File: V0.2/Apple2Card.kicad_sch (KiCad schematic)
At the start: 61 parts, among them J1 Conn_01x08_Pin, P2 Conn_02x13_Top_Bottom, Q2 2N3904, SW1 SW_DIP_x08, U1C1 74LS240, U1E1 74LS14, U2 74LS133, U2B1 74LS08, U2D1 74LS138, U2E1 74LS08, U3A1 2764, U3C1 ATF16V8C, U3D1 ATF16V8C, U3E1 74LS273/74HCT273, U4E1 74LS245, U5A1 NCR5380, U5C1 6264, U5E1 74LS14, U6C1 74LS32, U6D1 74LS74, U6E1 74LS74

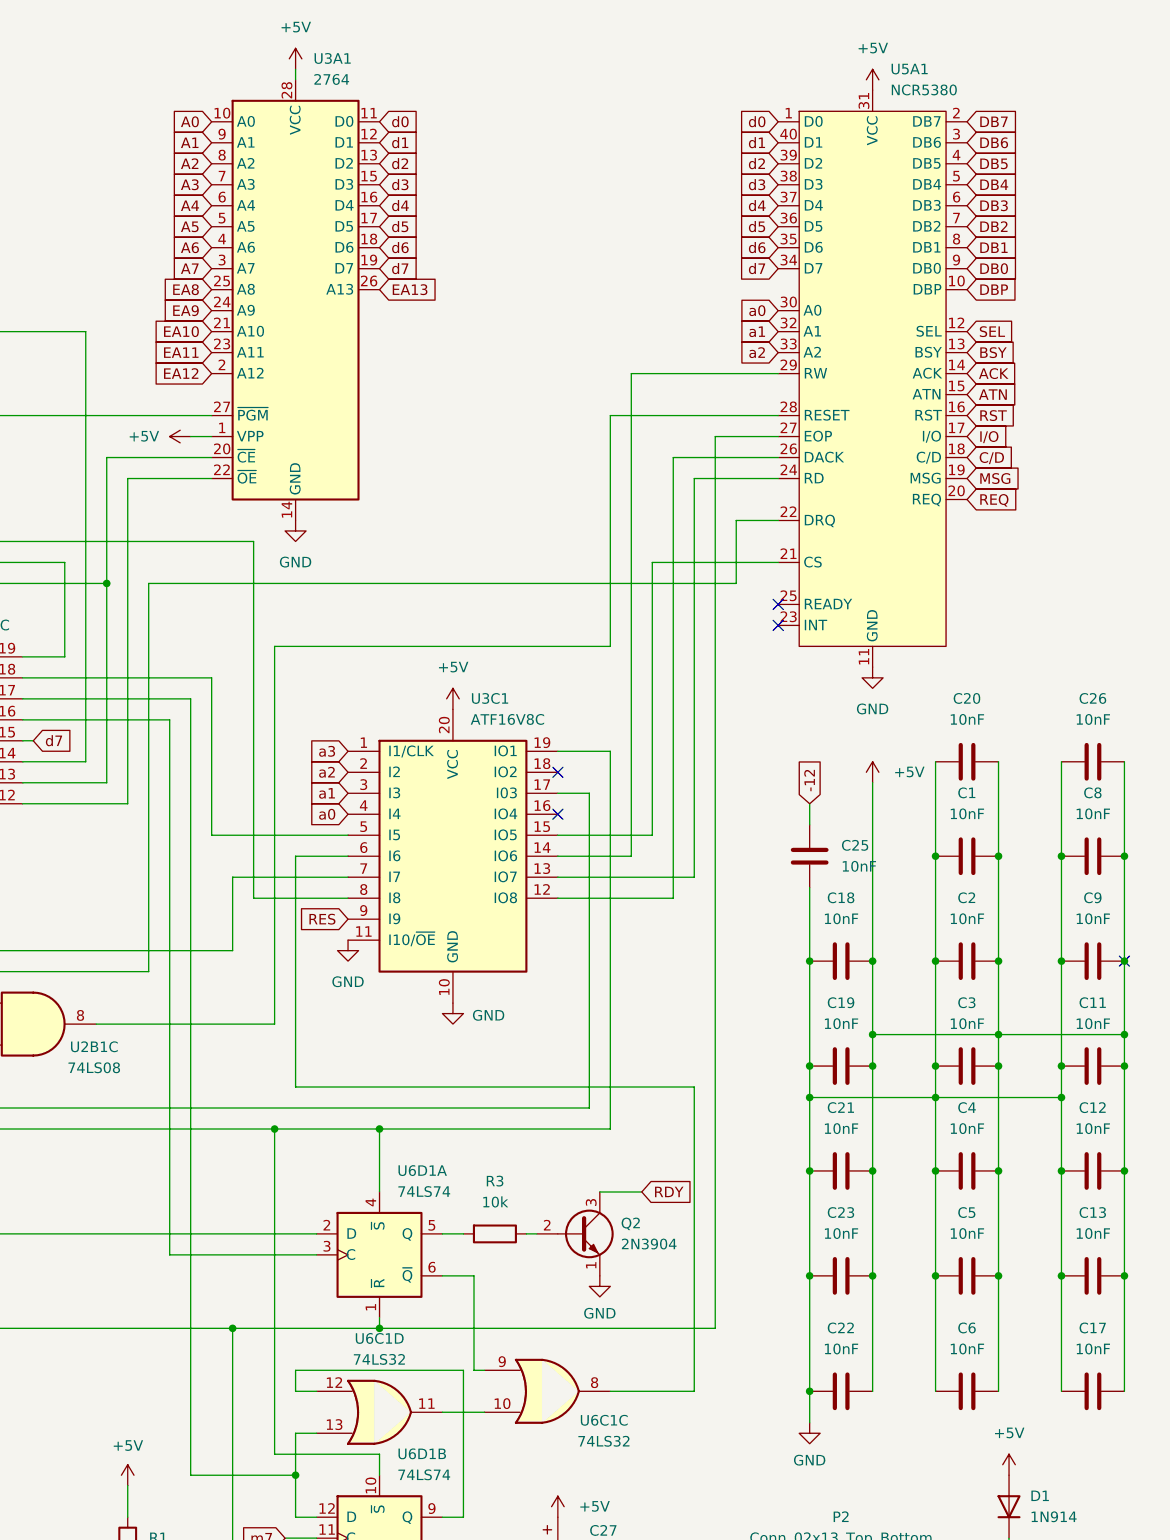
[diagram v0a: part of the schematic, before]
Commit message: menage
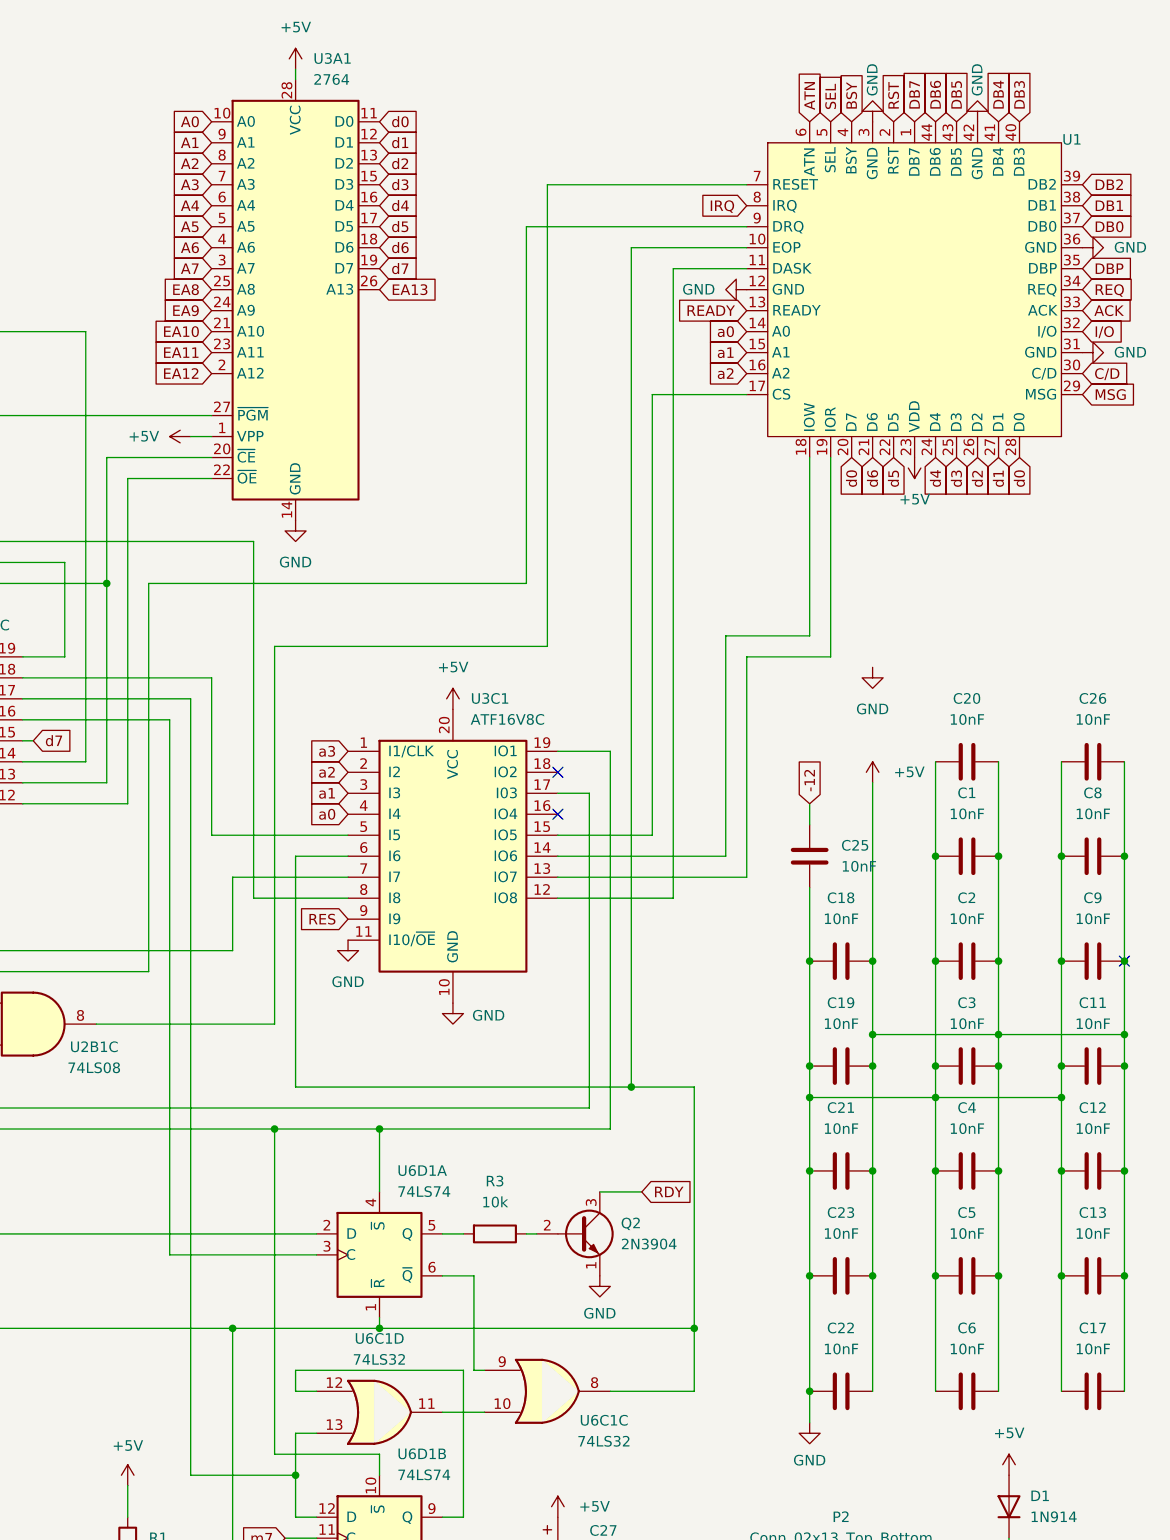
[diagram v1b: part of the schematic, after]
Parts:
- removed U5A1: NCR5380, Package_DIP:DIP-40_W15.24mm, symbol ncr5380:NCR5880
- added U1: ~, Package_LCC:PLCC-44, symbol 53c80:53c80_PLCC
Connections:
- net +5V: now also U1.23 (VDD)
- net ACK: now also U1.33 (ACK)
- net ATN: now also U1.6 (ATN)
- net BSY: now also U1.4 (BSY)
- net C/D: now also U1.30 (C/D)
- net DB0: now also U1.37 (DB0)
- net DB1: now also U1.38 (DB1)
- net DB2: now also U1.39 (DB2)
- net DB3: now also U1.40 (DB3)
- net DB4: now also U1.41 (DB4)
- net DB5: now also U1.43 (DB5)
- net DB6: now also U1.44 (DB6)
- net DB7: now also U1.1 (DB7)
- net DBP: now also U1.35 (DBP)
- net GND: now also U1.12 (GND), U1.3 (GND), U1.31 (GND), U1.36 (GND), U1.42 (GND)
- net IRQ: now also U1.8 (IRQ)
- net I/O: now also U1.32 (I/O)
- net MSG: now also U1.29 (MSG)
- net REQ: now also U1.34 (REQ)
- net RST: now also U1.2 (RST)
- net SEL: now also U1.5 (SEL)
- net a0: now also U1.14 (A0)
- net a1: now also U1.15 (A1)
- net a2: now also U1.16 (A2)
- net d0: now also U1.20 (D7), U1.28 (D0)
- net d1: now also U1.27 (D1)
- net d2: now also U1.26 (D2)
- net d3: now also U1.25 (D3)
- net d4: now also U1.24 (D4)
- net d5: now also U1.22 (D5)
- net d6: now also U1.21 (D6)
- net at R1.2, U6D1.1 (~{R}), U6D1.13 (~{R})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: now also U3C1.6 (I6), U6C1.8, U1.10 (EOP)
- net at U3C1.15 (IO5): now also U1.17 (CS)
- net at U3D1.9 (I9), U6D1.2 (D): now also U1.9 (DRQ)
- net at U3C1.13 (IO7): now also U1.19 (IOR)
- net at U3C1.12 (IO8): now also U1.11 (DASK)
- net at U2B1.8: now also U1.7 (RESET)
- net at U3C1.14 (IO6): now also U1.18 (IOW)
- new net READY: U1.13 (READY)
- no-connect marks 17 -> 15
